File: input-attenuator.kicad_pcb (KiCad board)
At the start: 2 copper layers, 100.1 x 56.4 mm, 44 parts, among them J1 DC_INTF, J2 RF_IN, J3 RX_1_RF, J4 RX_2_RF, K1 EE2-5TNU-L, K2 EE2-5TNU-L, K3 EE2-5TNU-L, K4 EE2-5TNU-L, Q1 MMBT3904, Q2 MMBT3904, Q3 MMBT3904, Q4 MMBT3904, Q5 MMBT3904, Q6 MMBT3904, Q7 MMBT3904, Q8 MMBT3904, U1 74HC595

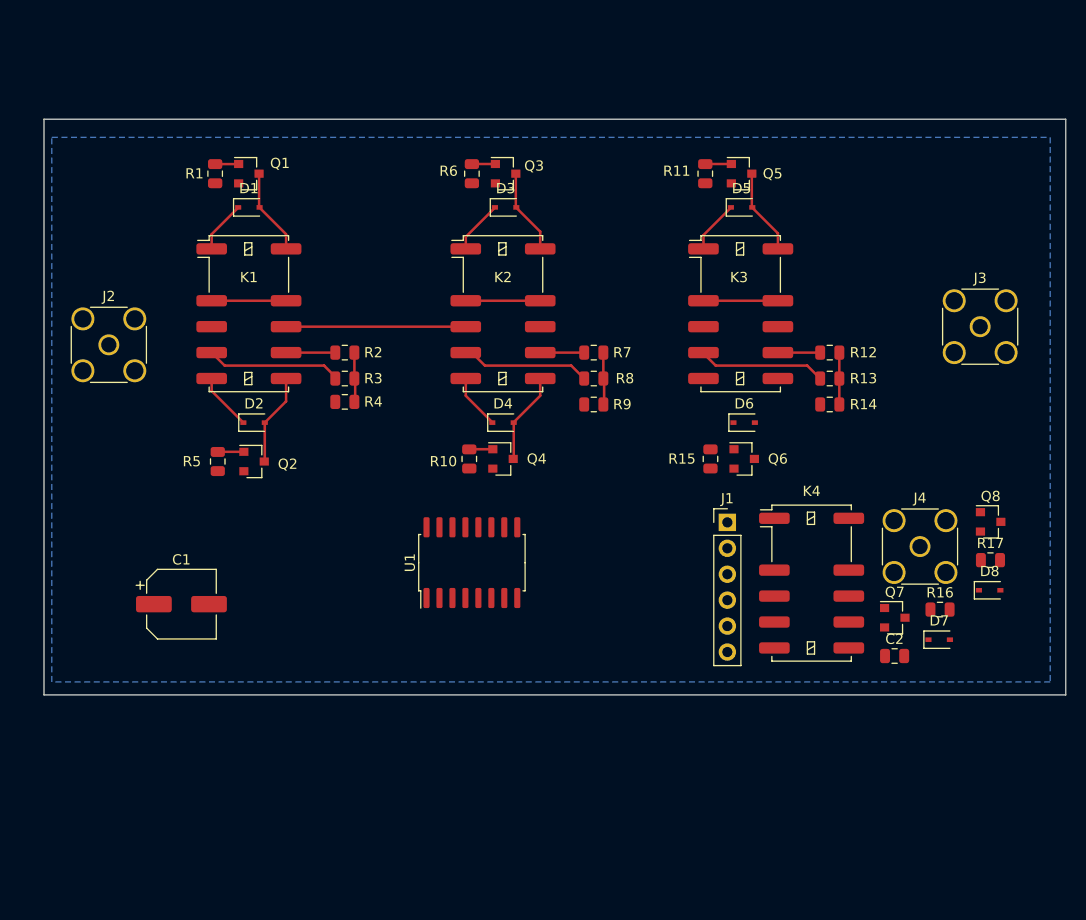
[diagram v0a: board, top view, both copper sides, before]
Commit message: relaysPlaced
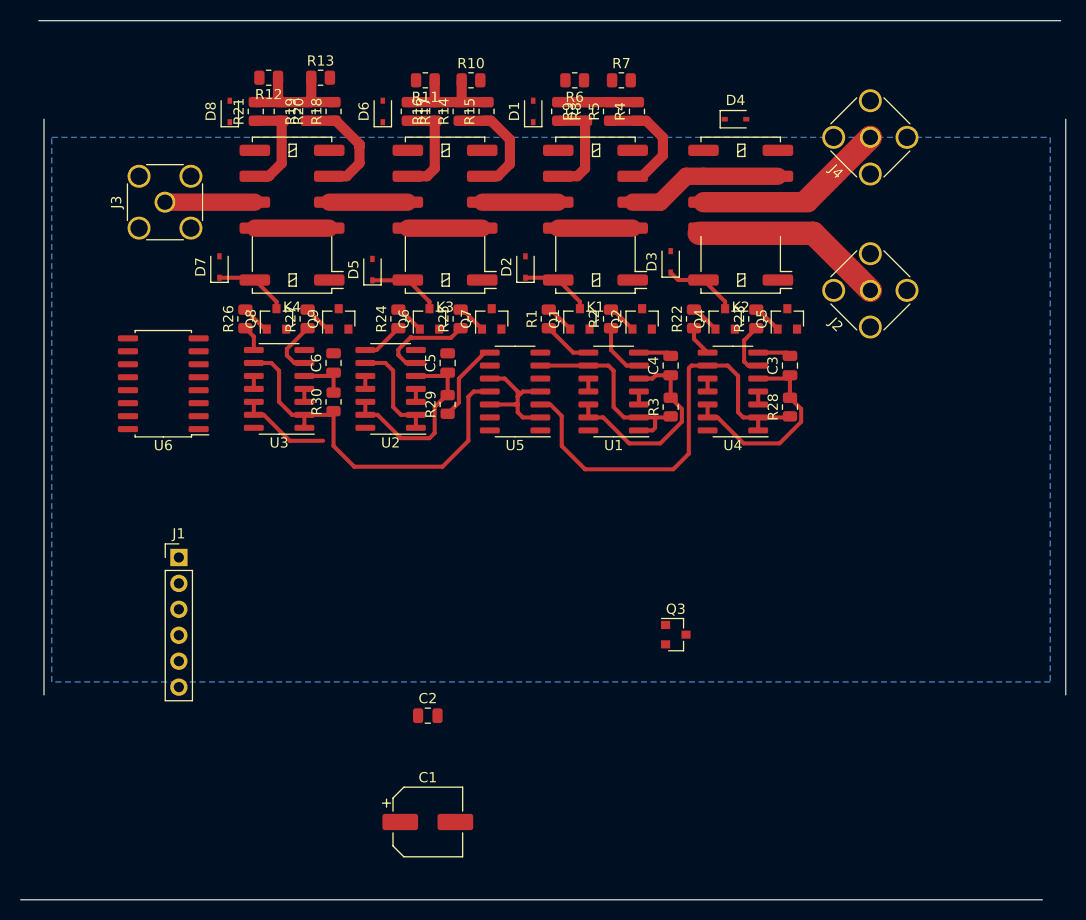
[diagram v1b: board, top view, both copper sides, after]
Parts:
- added C3: 0.22u, Capacitor_SMD:C_0805_2012Metric, F.Cu at (132.0, 56.6)
- added C4: 0.22u, Capacitor_SMD:C_0805_2012Metric, F.Cu at (120.3, 56.6)
- added C5: 0.22u, Capacitor_SMD:C_0805_2012Metric, F.Cu at (98.5, 56.4)
- added C6: 0.22u, Capacitor_SMD:C_0805_2012Metric, F.Cu at (87.3, 56.4)
- added Q9: BC858, Package_TO_SOT_SMD:SOT-23, F.Cu at (87.8, 52.1)
- added R18: _, Resistor_SMD:R_0805_2012Metric, F.Cu at (87.3, 31.8)
- added R19: 14.0_, Resistor_SMD:R_0805_2012Metric, F.Cu at (84.7, 31.8)
- added R20: 14.0_, Resistor_SMD:R_0805_2012Metric, F.Cu at (82.2, 31.8)
- added R21: _, Resistor_SMD:R_0805_2012Metric, F.Cu at (79.7, 31.8)
- added R22: 22K, Resistor_SMD:R_0805_2012Metric, F.Cu at (122.6, 52.1)
- added R23: 22K, Resistor_SMD:R_0805_2012Metric, F.Cu at (128.7, 52.1)
- added R24: 22K, Resistor_SMD:R_0805_2012Metric, F.Cu at (93.6, 52.1)
- added R25: 22K, Resistor_SMD:R_0805_2012Metric, F.Cu at (99.7, 52.1)
- added R26: 22K, Resistor_SMD:R_0805_2012Metric, F.Cu at (78.7, 52.1)
- added R27: 22K, Resistor_SMD:R_0805_2012Metric, F.Cu at (84.7, 52.1)
- added R28: 1M, Resistor_SMD:R_0805_2012Metric, F.Cu at (132.0, 60.7)
- added R29: 1M, Resistor_SMD:R_0805_2012Metric, F.Cu at (98.5, 60.5)
- added R30: 1M, Resistor_SMD:R_0805_2012Metric, F.Cu at (87.3, 60.2)
- added U2: 74HC00, Package_SO:SO-14_3.9x8.65mm_P1.27mm, F.Cu at (92.9, 58.9)
- added U3: 74HC00, Package_SO:SO-14_3.9x8.65mm_P1.27mm, F.Cu at (82.0, 58.9)
- added U4: 74HC00, Package_SO:SO-14_3.9x8.65mm_P1.27mm, F.Cu at (126.4, 59.2)
- added U5: 74HC00, Package_SO:SO-14_3.9x8.65mm_P1.27mm, F.Cu at (105.1, 59.2)
- added U6: 74HC595, Package_SO:SO-16_5.3x10.2mm_P1.27mm, F.Cu at (70.6, 58.4)
- Q1, Q2, Q4, Q5, Q6, Q7, Q8: value MMBT3904 -> BC858
- R10, R6: value 22K -> 82.2
- R11, R15, R16, R5: value 22K -> _
- R12: value 40.9 -> 82.2
- R13: value 40.9 -> _
- R14: value 10.1 -> 14.0_
- R17: value 22K -> 14.0_
- R2: value 14.0 -> 22K
- R3: value 14.0 -> 1M
- R4: value 82.2 -> 14.0_
- R7: value 26.0 -> _
- R8: value 26.0 -> 14.0_
- R9: value 35.1 -> _
- U1: value 74HC595 -> 74HC00; footprint Package_SO:SO-16_5.3x10.2mm_P1.27mm -> Package_SO:SO-14_3.9x8.65mm_P1.27mm
- moved D8 88.0 mm to (77.1, 31.8), turned to 90 degrees
- moved J3 80.8 mm to (70.8, 40.6), turned to 90 degrees
- moved D7 79.4 mm to (76.1, 47.0), turned to 90 degrees
- moved J2 74.8 mm to (139.9, 49.3), turned to 135 degrees
- moved Q8 72.7 mm to (81.7, 52.1), turned to 90 degrees
- moved R17 72.0 mm to (94.7, 31.8), turned to -90 degrees
- moved R16 69.5 mm to (97.2, 31.8), turned to 90 degrees
- moved K4 62.4 mm to (83.2, 41.9), turned to 180 degrees
- moved R12 61.2 mm to (80.9, 28.4)
- moved R13 57.9 mm to (86.0, 28.4)
- moved J1 53.8 mm to (72.1, 75.4)
- moved R5 51.6 mm to (114.5, 31.8)
- moved Q7 49.1 mm to (102.8, 52.1), turned to 90 degrees
- moved Q3 48.1 mm to (120.8, 83.0)
- moved D6 46.7 mm to (92.1, 31.8), turned to 90 degrees
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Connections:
- C1 pad 1: VRelay -> +5V
- C2 pad 2: VRelay -> +5V
- D1 pad 1: VRelay -> Net-(D1-Pad1)
- D1 pad 2: Net-(D1-Pad2) -> GND
- D2 pad 1: VRelay -> Net-(D2-Pad1)
- D2 pad 2: Net-(D2-Pad2) -> GND
- D3 pad 1: VRelay -> Net-(D3-Pad1)
- D3 pad 2: Net-(D3-Pad2) -> GND
- D4 pad 1: VRelay -> Net-(D4-Pad1)
- D4 pad 2: Net-(D4-Pad2) -> GND
- D5 pad 1: VRelay -> Net-(D5-Pad1)
- D5 pad 2: Net-(D5-Pad2) -> GND
- D6 pad 1: VRelay -> Net-(D6-Pad1)
- D6 pad 2: Net-(D6-Pad2) -> GND
- D7 pad 1: VRelay -> Net-(D7-Pad1)
- D7 pad 2: Net-(D7-Pad2) -> GND
- D8 pad 1: VRelay -> Net-(D8-Pad1)
- D8 pad 2: Net-(D8-Pad2) -> GND
- J1 pad 1: VRelay -> +5V
- J2 pad 1: RF_IN -> /RF_TX
- J3 pad 1: RX_1_RF -> /RF_RX
- J4 pad 1: RX_2_RF -> /Antenna
- K1 pad 1: VRelay -> GND
- K1 pad 12: Net-(D1-Pad2) -> Net-(D2-Pad1)
- K1 pad 4: RF_IN -> Net-(K1-Pad4)
- K1 pad 6: VRelay -> GND
- K1 pad 7: Net-(D2-Pad2) -> Net-(D1-Pad1)
- K2 pad 1: VRelay -> GND
- K2 pad 10: Net-(K2-Pad10) -> /RF_TX
- K2 pad 12: Net-(D3-Pad2) -> Net-(D3-Pad1)
- K2 pad 3: Net-(K2-Pad10) -> /RF_TX
- K2 pad 4: Net-(K1-Pad9) -> /Antenna
- K2 pad 5: Net-(K2-Pad5) -> Net-(K1-Pad4)
- K2 pad 6: VRelay -> GND
- K2 pad 7: Net-(D4-Pad2) -> Net-(D4-Pad1)
- K2 pad 8: Net-(K2-Pad8) -> Net-(K1-Pad4)
- K2 pad 9: Net-(K2-Pad9) -> /Antenna
- K3 pad 1: VRelay -> GND
- K3 pad 12: Net-(D5-Pad2) -> Net-(D5-Pad1)
- K3 pad 4: Net-(K2-Pad9) -> Net-(K1-Pad9)
- K3 pad 6: VRelay -> GND
- K3 pad 7: Net-(D6-Pad2) -> Net-(D6-Pad1)
- K4 pad 1: VRelay -> GND
- K4 pad 10: GND -> Net-(K4-Pad10)
- K4 pad 12: Net-(D7-Pad2) -> Net-(D7-Pad1)
- K4 pad 3: Net-(K3-Pad9) -> Net-(K4-Pad10)
- K4 pad 4: RX_1_RF -> Net-(K3-Pad9)
- K4 pad 5: GND -> Net-(K4-Pad5)
- K4 pad 6: VRelay -> GND
- K4 pad 7: Net-(D8-Pad2) -> Net-(D8-Pad1)
- K4 pad 8: Net-(K3-Pad9) -> Net-(K4-Pad8)
- K4 pad 9: RX_2_RF -> /RF_RX
- Q1 pad 2: GND -> +5V
- Q1 pad 3: Net-(D1-Pad2) -> Net-(D2-Pad1)
- Q2 pad 2: GND -> +5V
- Q2 pad 3: Net-(D2-Pad2) -> Net-(D1-Pad1)
- Q3 pad 1: Net-(Q3-Pad1) -> unconnected-(Q3-Pad1)
- Q3 pad 2: GND -> unconnected-(Q3-Pad2)
- Q3 pad 3: Net-(D3-Pad2) -> unconnected-(Q3-Pad3)
- Q4 pad 2: GND -> +5V
- Q4 pad 3: Net-(D4-Pad2) -> Net-(D3-Pad1)
- Q5 pad 2: GND -> +5V
- Q5 pad 3: Net-(D5-Pad2) -> Net-(D4-Pad1)
- Q6 pad 2: GND -> +5V
- Q6 pad 3: Net-(D6-Pad2) -> Net-(D5-Pad1)
- Q7 pad 2: GND -> +5V
- Q7 pad 3: Net-(D7-Pad2) -> Net-(D6-Pad1)
- Q8 pad 2: GND -> +5V
- Q8 pad 3: Net-(D8-Pad2) -> Net-(D7-Pad1)
- R1 pad 1: A1_ON -> Net-(R1-Pad1)
- R10 pad 1: A2_OFF -> Net-(R10-Pad1)
- R10 pad 2: Net-(Q4-Pad1) -> GND
- R11 pad 1: A3_ON -> Net-(R10-Pad1)
- R11 pad 2: Net-(Q5-Pad1) -> GND
- R12 pad 2: Net-(K3-Pad8) -> GND
- R13 pad 1: Net-(K3-Pad5) -> Net-(R12-Pad1)
- R13 pad 2: Net-(R12-Pad1) -> GND
- R14 pad 1: Net-(R12-Pad1) -> Net-(K3-Pad5)
- R14 pad 2: GND -> Net-(R10-Pad1)
- R15 pad 1: A3_OFF -> Net-(K3-Pad5)
- R15 pad 2: Net-(Q6-Pad1) -> Net-(R10-Pad1)
- R16 pad 1: RX_1_ON -> Net-(K3-Pad8)
- R16 pad 2: Net-(Q7-Pad1) -> Net-(R10-Pad1)
- R17 pad 1: RX_2_ON -> Net-(R10-Pad1)
- R17 pad 2: Net-(Q8-Pad1) -> Net-(K3-Pad8)
- R2 pad 2: Net-(K1-Pad8) -> Net-(Q2-Pad1)
- R3 pad 1: Net-(K1-Pad5) -> Net-(R3-Pad1)
- R3 pad 2: Net-(R2-Pad1) -> Net-(R3-Pad2)
- R4 pad 1: Net-(R2-Pad1) -> Net-(K1-Pad5)
- R4 pad 2: GND -> Net-(R4-Pad2)
- R5 pad 1: A1_OFF -> Net-(K1-Pad5)
- R5 pad 2: Net-(Q2-Pad1) -> Net-(R4-Pad2)
- R6 pad 1: A2_ON -> Net-(R4-Pad2)
- R6 pad 2: Net-(Q3-Pad1) -> GND
- R7 pad 1: Net-(R7-Pad1) -> Net-(R4-Pad2)
- R7 pad 2: Net-(K2-Pad8) -> GND
- R8 pad 1: Net-(K2-Pad5) -> Net-(R4-Pad2)
- R8 pad 2: Net-(R7-Pad1) -> Net-(K1-Pad8)
- R9 pad 1: Net-(R7-Pad1) -> Net-(K1-Pad8)
- R9 pad 2: GND -> Net-(R4-Pad2)
- U1 pad 1: A1_OFF -> Net-(R3-Pad1)
- U1 pad 10: VRelay -> Net-(U1-Pad10)
- U1 pad 11: Net-(J1-Pad4) -> Net-(U1-Pad10)
- U1 pad 12: Net-(J1-Pad5) -> Net-(R3-Pad2)
- U1 pad 13: GND -> Net-(R3-Pad2)
- U1 pad 14: Net-(J1-Pad3) -> +5V
- U1 pad 2: A2_ON -> Net-(R3-Pad1)
- U1 pad 3: A2_OFF -> Net-(U1-Pad3)
- U1 pad 4: A3_ON -> Net-(U1-Pad3)
- U1 pad 5: A3_OFF -> Net-(R3-Pad2)
- U1 pad 6: RX_1_ON -> Net-(R2-Pad1)
- U1 pad 7: RX_2_ON -> GND
- U1 pad 8: GND -> Net-(R1-Pad1)
- U1 pad 9: Net-(J1-Pad6) -> Net-(R3-Pad1)
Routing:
- net Net-(U4-Pad1): track 0.00 -> 43.4 mm
- net Net-(R30-Pad1): track 0.00 -> 38.2 mm
- net VRelay: track 26.6 -> 0.00 mm
- net /Antenna: track 0.00 -> 21.8 mm
- net Net-(R3-Pad2): track 0.00 -> 20.6 mm
- net Net-(C3-Pad1): track 0.00 -> 20.6 mm
- net Net-(R3-Pad1): track 0.00 -> 19.9 mm
- net /RF_TX: track 0.00 -> 19.1 mm
- net Net-(C5-Pad1): track 0.00 -> 19.0 mm
- net Net-(R29-Pad1): track 0.00 -> 18.4 mm
- net Net-(K1-Pad4): track 0.00 -> 15.3 mm
- net Net-(C6-Pad1): track 0.00 -> 14.1 mm
- net powerDown: track 0.00 -> 13.1 mm
- net Net-(K2-Pad5): track 12.6 -> 0.00 mm
- net Net-(R10-Pad1): track 0.00 -> 11.9 mm
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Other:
- board size 100.1 x 56.4 mm -> 102.4 x 86.1 mm
